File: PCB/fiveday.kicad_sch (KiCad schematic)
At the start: 55 parts, among them SW1 SW_PUSH, SW10 SW_PUSH, SW11 SW_PUSH, SW12 SW_PUSH, SW13 SW_PUSH, SW14 SW_PUSH, SW15 SW_PUSH, SW16 SW_PUSH, SW18 SW_PUSH, SW19 SW_PUSH, SW2 SW_PUSH, SW20 SW_PUSH, SW21 SW_PUSH, SW22 SW_PUSH, SW23 SW_PUSH, SW24 SW_PUSH, SW25 SW_PUSH, SW26 SW_PUSH, SW27 SW_PUSH, SW28 SW_PUSH, SW29 SW_PUSH, SW3 SW_PUSH, SW30 SW_PUSH, SW31 SW_PUSH, SW32 SW_PUSH, SW33 SW_PUSH, SW34 SW_PUSH, SW35 SW_PUSH, SW36 SW_PUSH, SW37 SW_PUSH, SW38 SW_PUSH, SW39 SW_PUSH, SW4 SW_PUSH, SW40 SW_PUSH, SW41 SW_PUSH, SW42 SW_PUSH, SW43 SW_PUSH, SW44 SW_PUSH, SW45 SW_PUSH, SW46 SW_PUSH, SW47 SW_PUSH, SW48 SW_PUSH, SW49 SW_PUSH, SW5 SW_PUSH, SW50 SW_PUSH, SW51 SW_PUSH, SW52 SW_PUSH, SW53 SW_PUSH, SW54 SW_PUSH, SW55 SW_PUSH, SW6 SW_PUSH, SW7 SW_PUSH, SW8 SW_PUSH, SW9 SW_PUSH, U1 RP2040-ZERO

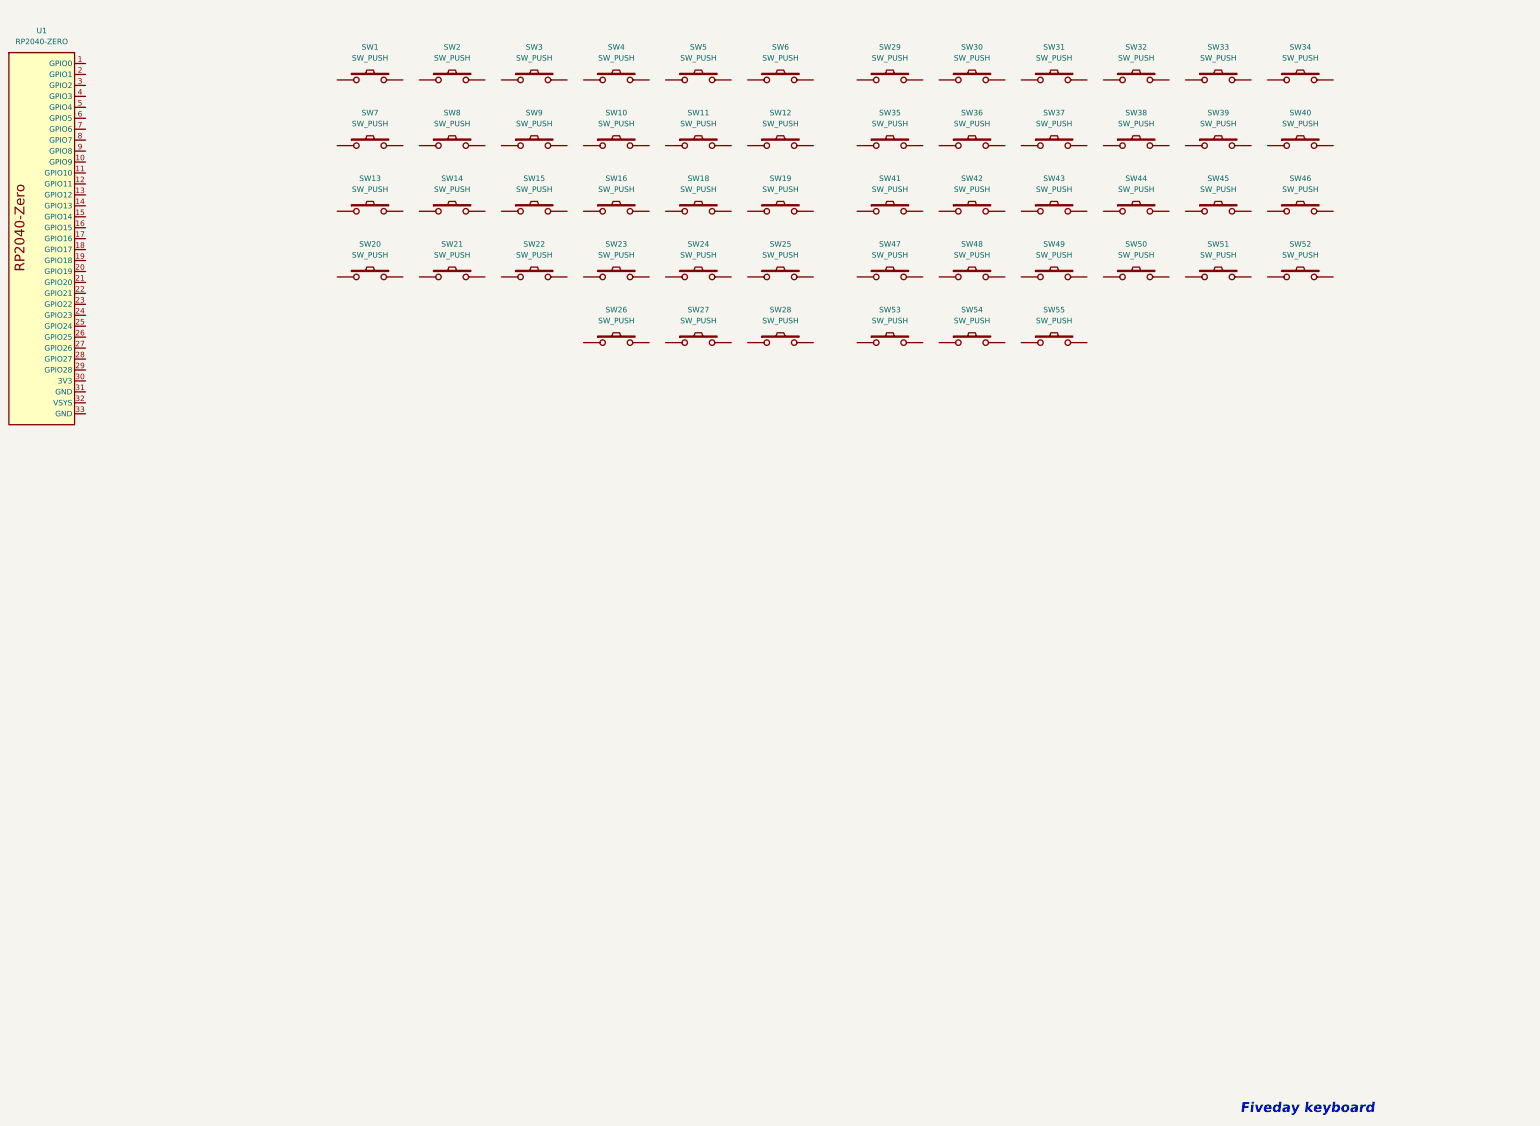
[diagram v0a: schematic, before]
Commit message: Better switch symbols
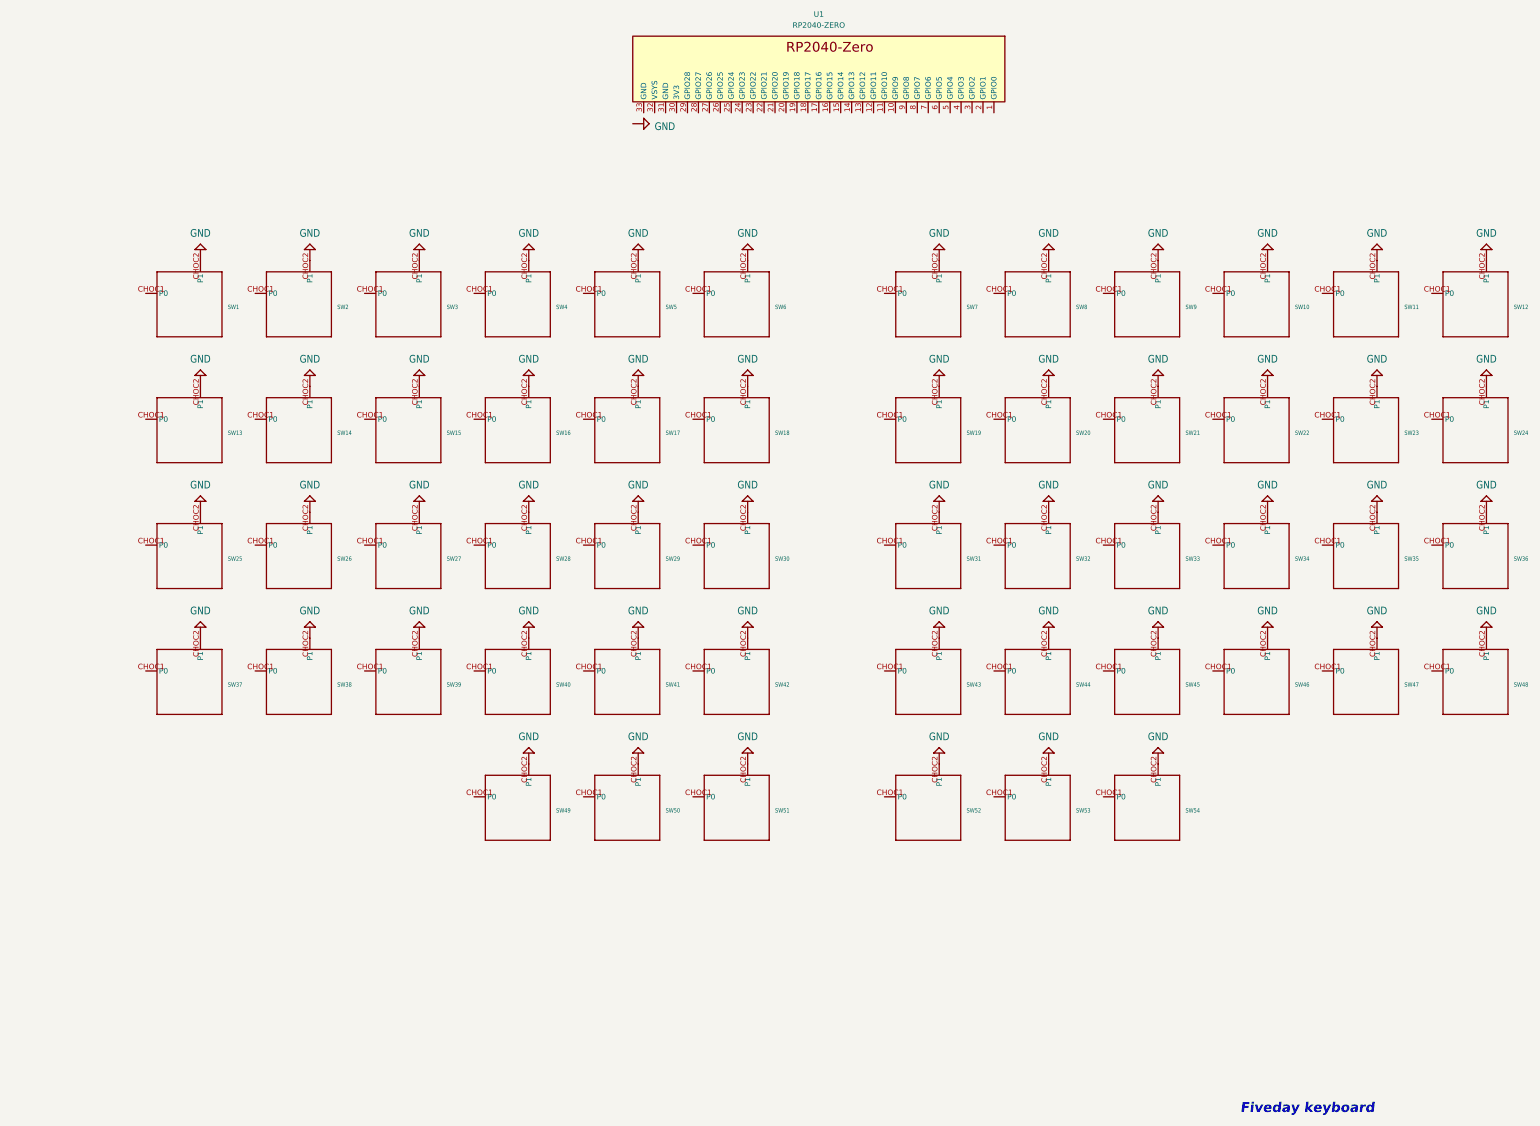
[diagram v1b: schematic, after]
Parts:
- removed SW1, SW10, SW11, SW12, SW13, SW14, SW15, SW16, SW18, SW19, SW2, SW20, SW21, SW22, SW23, SW24, SW25, SW26, SW27, SW28, SW29, SW3, SW30, SW31, SW32, SW33, SW34, SW35, SW36, SW37, SW38, SW39, SW4, SW40, SW41, SW42, SW43, SW44, SW45, SW46, SW47, SW48, SW49, SW5, SW50, SW51, SW52, SW53, SW54, SW55, SW6, SW7, SW8, SW9: SW_PUSH, symbol SofleKeyboard-rescue:SW_PUSH
- added SW1, SW10, SW11, SW12, SW13, SW14, SW15, SW16, SW17, SW18, SW19, SW2, SW20, SW21, SW22, SW23, SW24, SW25, SW26, SW27, SW28, SW29, SW3, SW30, SW31, SW32, SW33, SW34, SW35, SW36, SW37, SW38, SW39, SW4, SW40, SW41, SW42, SW43, SW44, SW45, SW46, SW47, SW48, SW49, SW5, SW50, SW51, SW52, SW53, SW54, SW6, SW7, SW8, SW9: KEYSWITCH-PLAIN-CHOC--6U, symbol Cyberdeck Mech Keeb-eagle-import:KEYSWITCH-PLAIN-CHOC--6U
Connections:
- new net GND: SW1.CHOC2 (P1), SW10.CHOC2 (P1), SW11.CHOC2 (P1), SW12.CHOC2 (P1), SW13.CHOC2 (P1), SW14.CHOC2 (P1), SW15.CHOC2 (P1), SW16.CHOC2 (P1), SW17.CHOC2 (P1), SW18.CHOC2 (P1), SW19.CHOC2 (P1), SW2.CHOC2 (P1), SW20.CHOC2 (P1), SW21.CHOC2 (P1), SW22.CHOC2 (P1), SW23.CHOC2 (P1), SW24.CHOC2 (P1), SW25.CHOC2 (P1), SW26.CHOC2 (P1), SW27.CHOC2 (P1), SW28.CHOC2 (P1), SW29.CHOC2 (P1), SW3.CHOC2 (P1), SW30.CHOC2 (P1), SW31.CHOC2 (P1), SW32.CHOC2 (P1), SW33.CHOC2 (P1), SW34.CHOC2 (P1), SW35.CHOC2 (P1), SW36.CHOC2 (P1), SW37.CHOC2 (P1), SW38.CHOC2 (P1), SW39.CHOC2 (P1), SW4.CHOC2 (P1), SW40.CHOC2 (P1), SW41.CHOC2 (P1), SW42.CHOC2 (P1), SW43.CHOC2 (P1), SW44.CHOC2 (P1), SW45.CHOC2 (P1), SW46.CHOC2 (P1), SW47.CHOC2 (P1), SW48.CHOC2 (P1), SW49.CHOC2 (P1), SW5.CHOC2 (P1), SW50.CHOC2 (P1), SW51.CHOC2 (P1), SW52.CHOC2 (P1), SW53.CHOC2 (P1), SW54.CHOC2 (P1), SW6.CHOC2 (P1), SW7.CHOC2 (P1), SW8.CHOC2 (P1), SW9.CHOC2 (P1)
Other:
- moved on the sheet: U1
